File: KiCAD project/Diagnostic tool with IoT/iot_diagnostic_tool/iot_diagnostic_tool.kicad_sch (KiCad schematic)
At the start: 15 parts, among them SW1 SW_Push, SW2 BOOT, U1 STM32L431RCTx, Y1 16 MHz

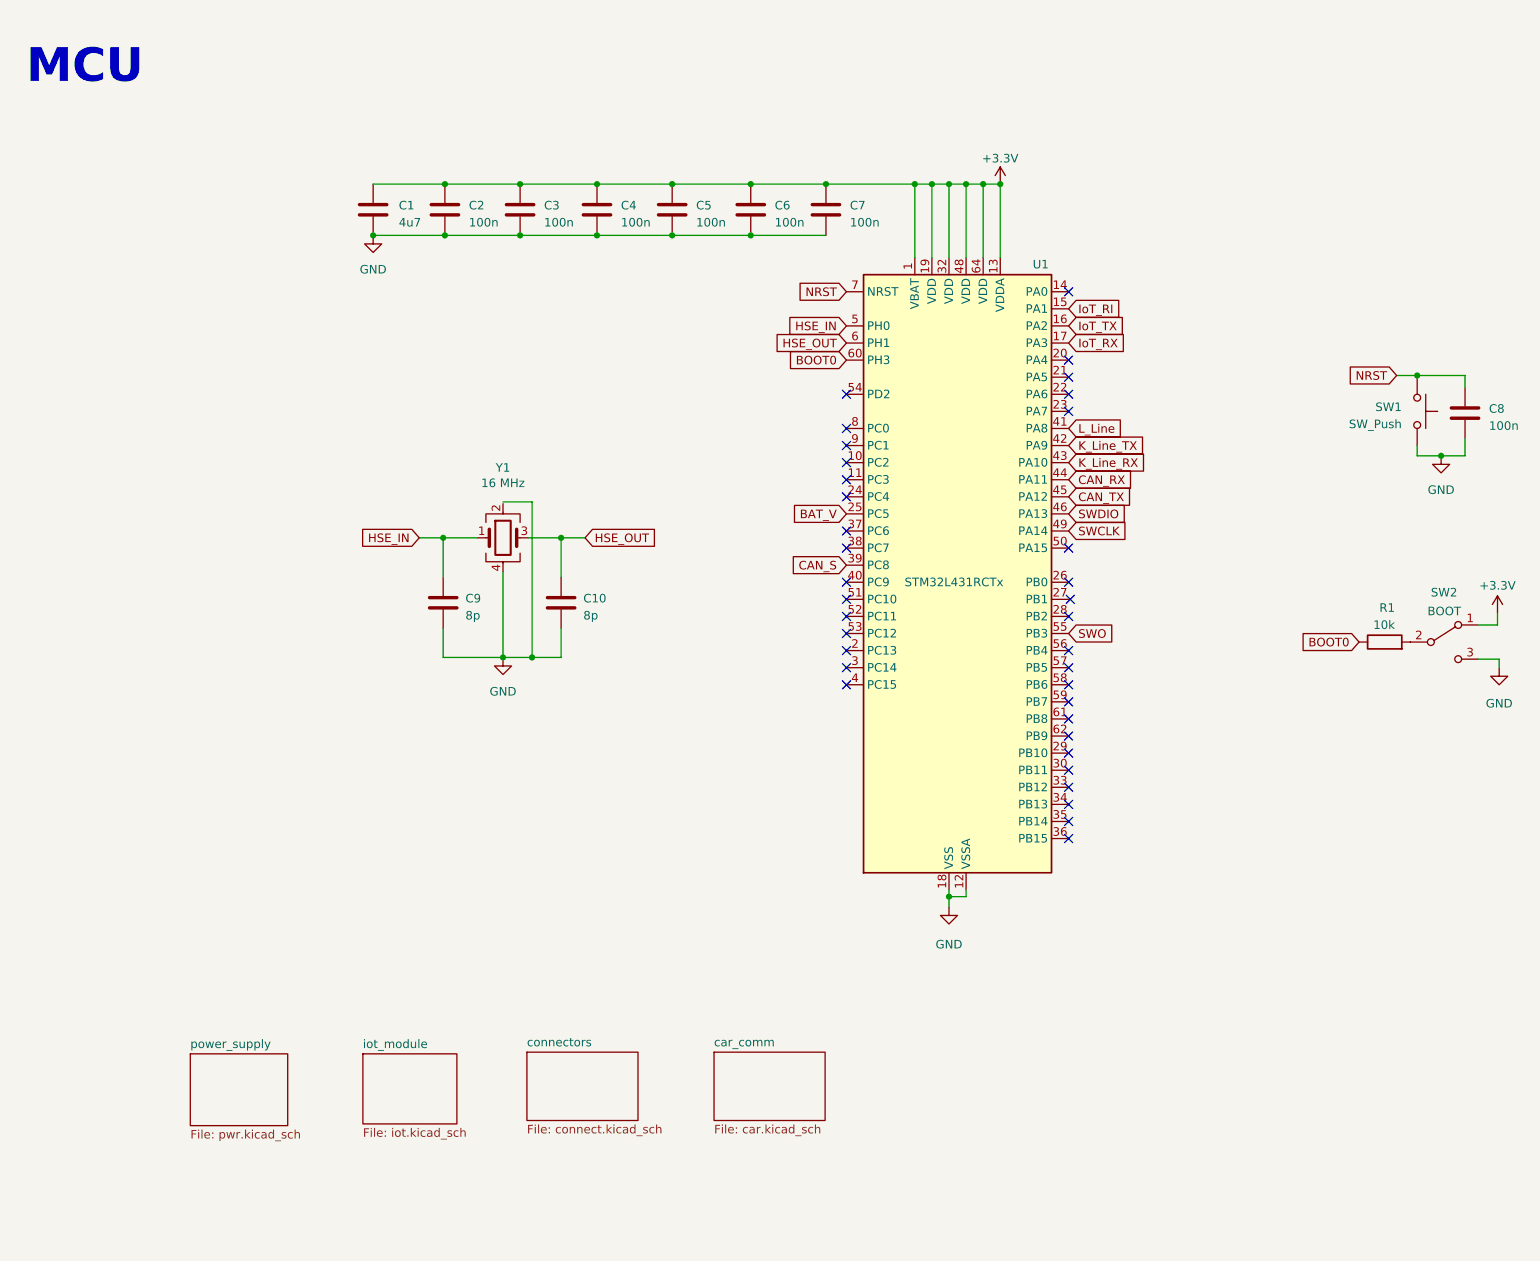
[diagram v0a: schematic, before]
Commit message: Update 03/03/23 - new schematic done
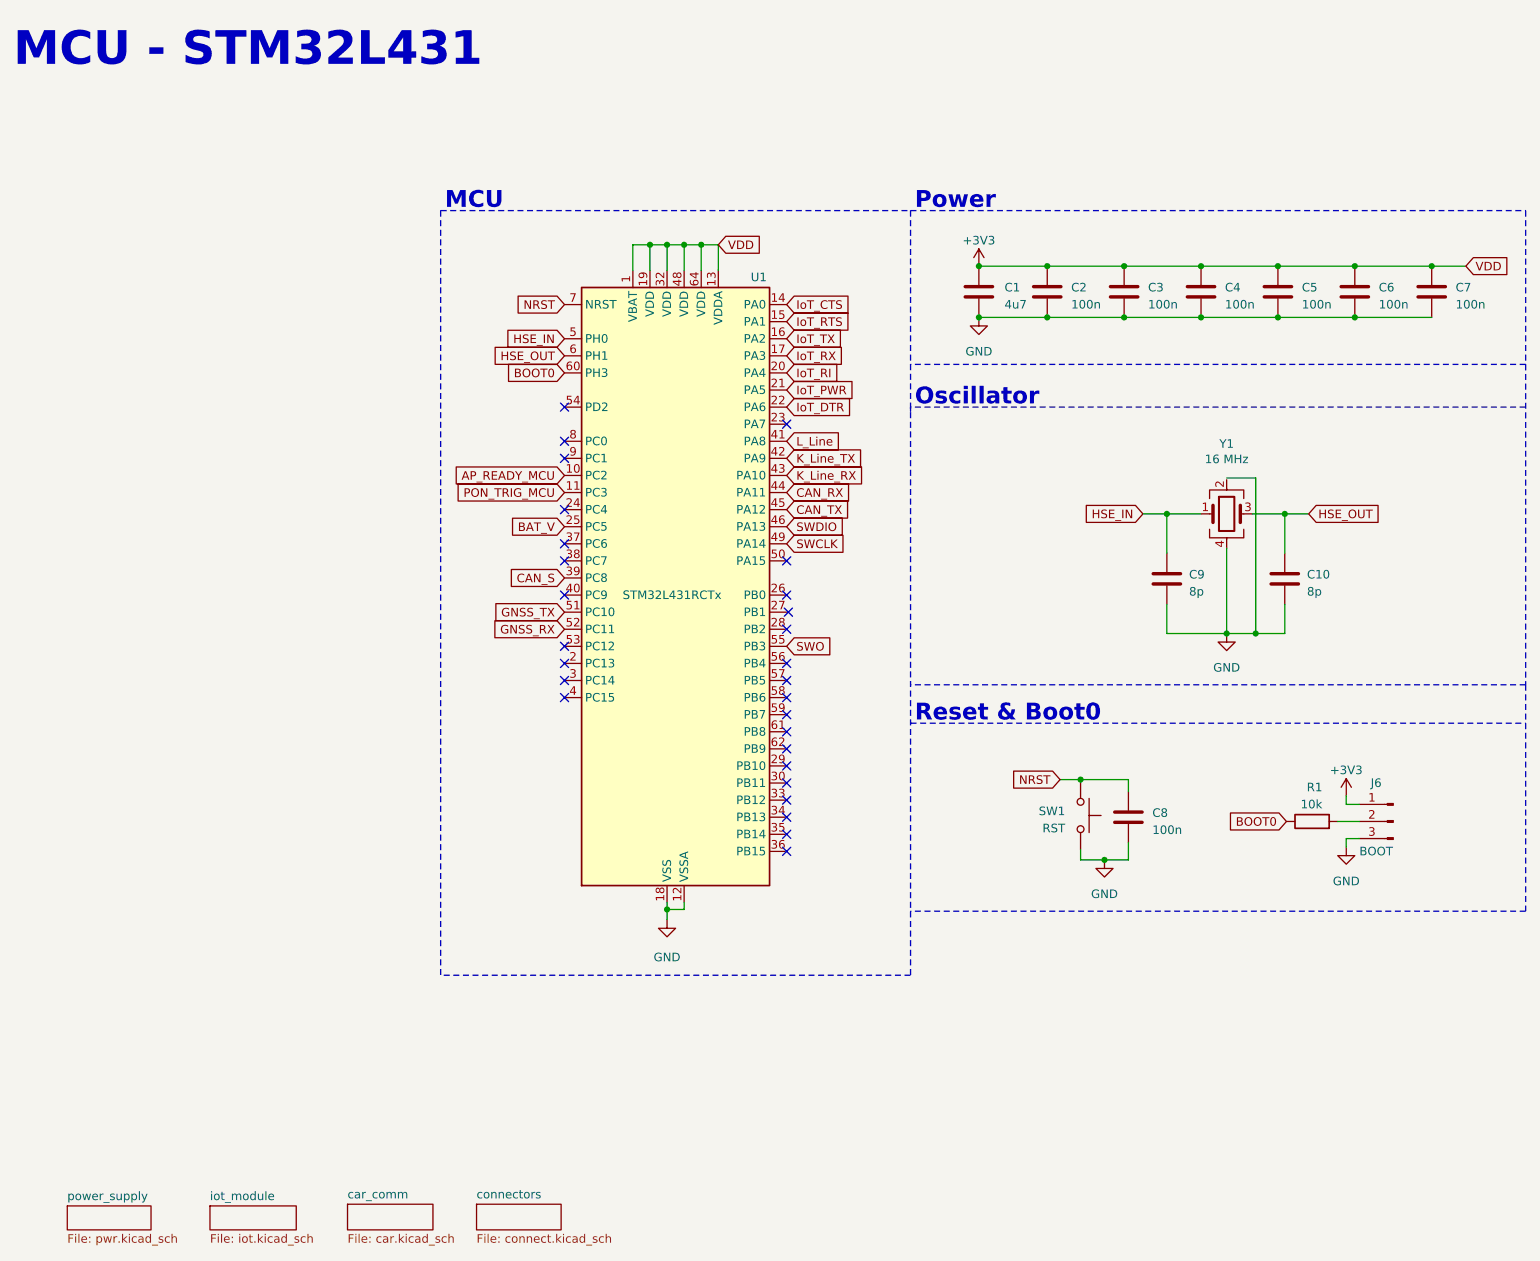
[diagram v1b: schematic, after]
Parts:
- removed SW2: BOOT, symbol Switch:SW_SPDT
- added J6: BOOT, symbol Connector:Conn_01x03_Pin
- SW1: value SW_Push -> RST
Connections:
- net GND: now also J6.3 (Pin_3)
- net IoT_RI: now also U1.20 (PA4); no longer U1.15 (PA1)
- net AP_READY_MCU: now reaches U1.10 (PC2)
- net PON_TRIG_MCU: now reaches U1.11 (PC3)
- net IoT_CTS: now reaches U1.14 (PA0)
- net IoT_PWR: now reaches U1.21 (PA5)
- net IoT_DTR: now reaches U1.22 (PA6)
- net GNSS_TX: now reaches U1.51 (PC10)
- net GNSS_RX: now reaches U1.52 (PC11)
- net at R1.2: now also J6.2 (Pin_2)
- net +3.3V renamed +3V3
- net +3V3: now also J6.1 (Pin_1)
- new net IoT_RTS: U1.15 (PA1)
- no-connect marks 36 -> 28
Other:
- note added: "MCU - STM32L431"
- note added: "Oscillator"
- note added: "Power"
- note added: "Reset & Boot0"
- moved on the sheet: C1, C10, C2, C3, C4, C5, C6, C7, C8, C9, R1, SW1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
